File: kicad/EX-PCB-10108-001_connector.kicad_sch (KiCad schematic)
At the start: 61 parts, among them CN1 PV-EC-CON-008-014, CN2 PV-EC-CON-013-006, CN3 PV-EC-CON-008-014, CN4 PV-EC-CON-010-010, CN5 PV-EC-CON-012-003, CN6 PV-EC-CON-010-004, J1 Conn_02x02_Odd_Even, U2 PV-EC-PTN-004-004, U3 PV-EC-PTN-004-001, U7 PV-EC-PTN-004-001, U8 PV-EC-PTN-004-001

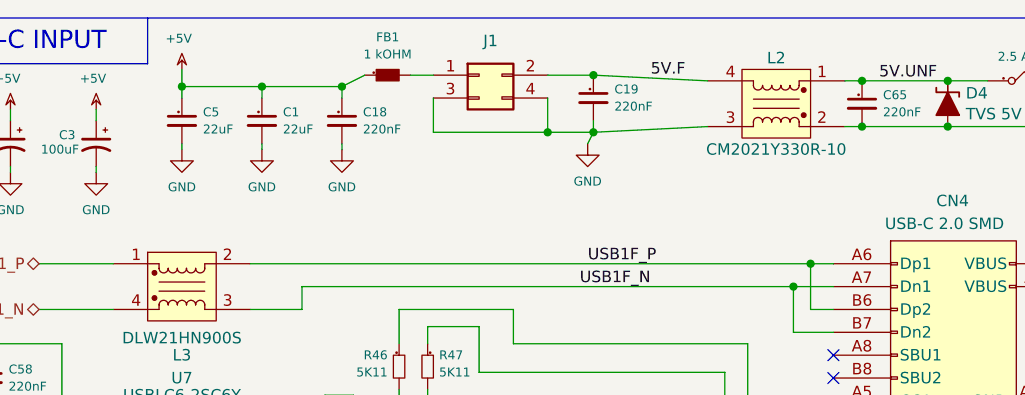
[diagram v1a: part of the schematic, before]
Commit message: touch up sch
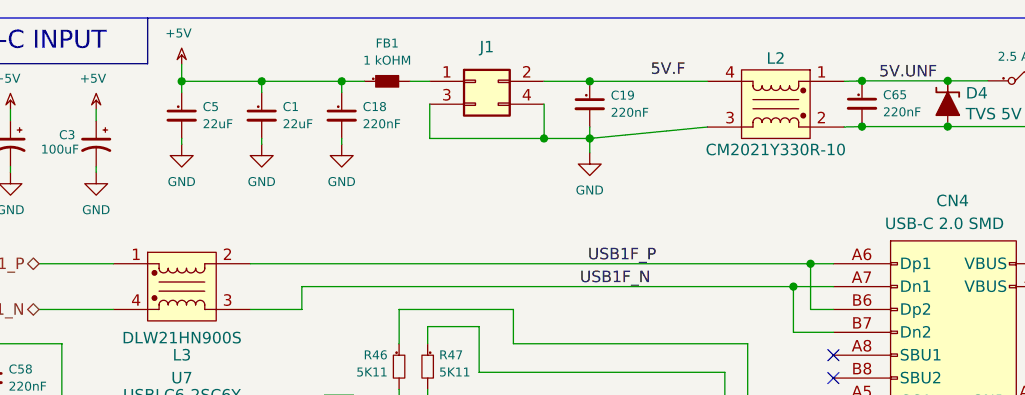
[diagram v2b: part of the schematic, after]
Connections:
- net 5V.F: no longer C19.1, J1.2 (Pin_2), L2.4
- new net: C19.1, J1.2 (Pin_2), L2.4
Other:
- moved on the sheet: C1, C18, C19, C5, FB1, J1
